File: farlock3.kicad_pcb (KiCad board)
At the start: 2 copper layers, 53 x 17.8 mm, 38 parts, among them J1 USB_B_Micro, J2 Conn_01x17, SW1 SW_SPDT, U1 MDBT50Q, U2 MX25R6435FZNIL0, U3 TB6612FNG, U4 AP2112K-3.3, Y1 32.768kHz

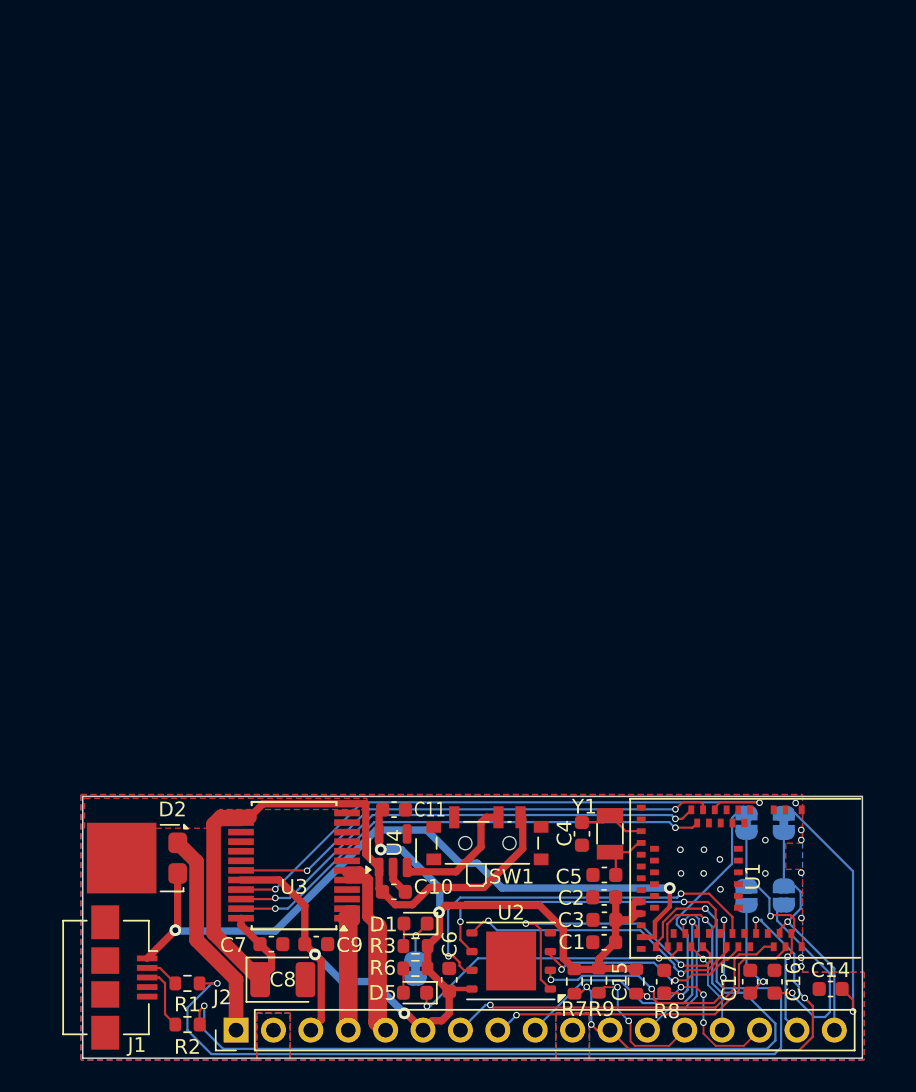
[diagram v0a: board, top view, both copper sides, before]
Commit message: v02 redesign
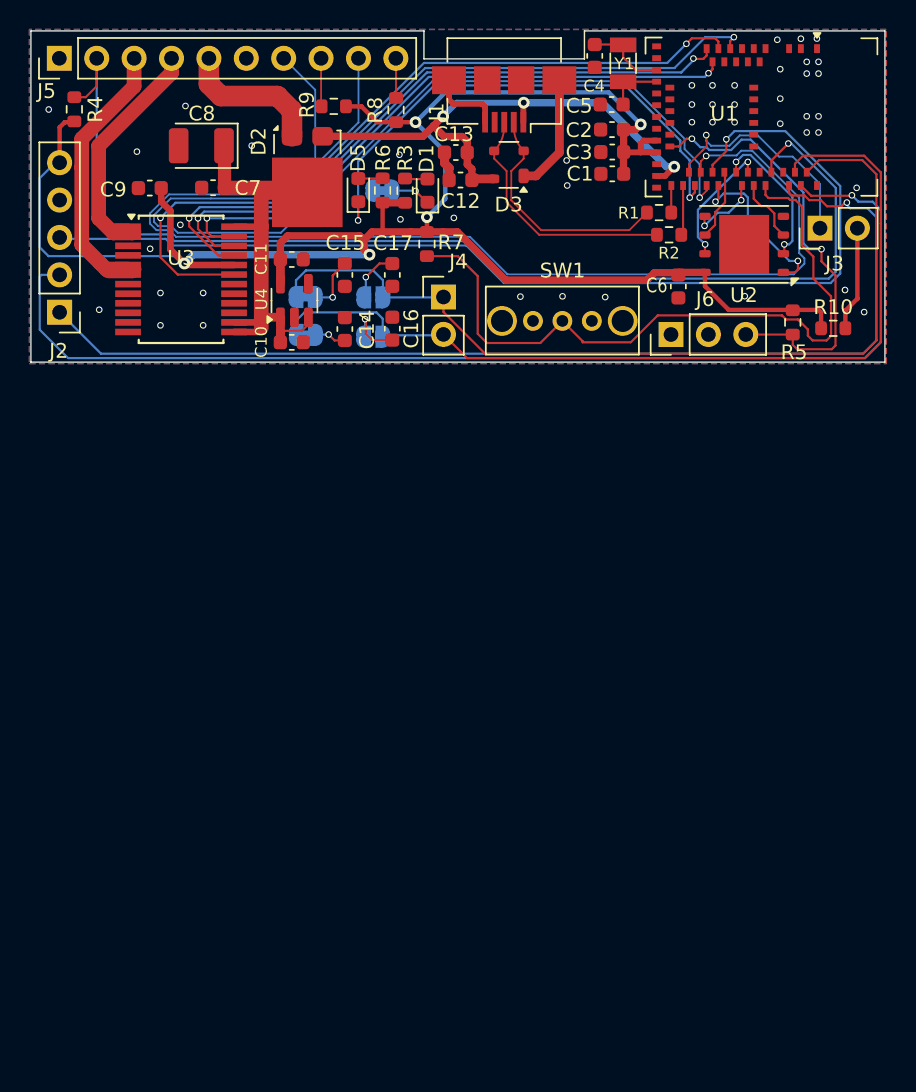
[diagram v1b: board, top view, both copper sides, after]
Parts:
- added C12: 10µF, Capacitor_SMD:C_0603_1608Metric, F.Cu at (155.6, 85.1)
- added C13: 0.1µF, Capacitor_SMD:C_0603_1608Metric, F.Cu at (155.3, 83.3)
- added D3: PRTR5V0U2X, Package_TO_SOT_SMD:SOT-143, F.Cu at (158.9, 84.1)
- added J3: Conn_01x02, Connector_PinHeader_2.54mm:PinHeader_1x02_P2.54mm_Vertical, F.Cu at (180.0, 88.4)
- added J4: Conn_01x02, Connector_PinHeader_2.54mm:PinHeader_1x02_P2.54mm_Vertical, F.Cu at (154.4, 93.1)
- added J5: Conn_01x10, Connector_PinHeader_2.54mm:PinHeader_1x10_P2.54mm_Vertical, F.Cu at (128.3, 76.9)
- added J6: Conn_01x03, Connector_PinHeader_2.54mm:PinHeader_1x03_P2.54mm_Vertical, F.Cu at (169.9, 95.6)
- added R10: 330, Resistor_SMD:R_0603_1608Metric, F.Cu at (180.9, 95.2)
- added R4: 10k, Resistor_SMD:R_0603_1608Metric, F.Cu at (129.3, 80.3)
- added R5: 10k, Resistor_SMD:R_0603_1608Metric, F.Cu at (178.2, 94.8)
- J2: value Conn_01x17 -> Conn_01x05; footprint Connector_PinHeader_2.54mm:PinHeader_1x17_P2.54mm_Vertical -> Connector_PinHeader_2.54mm:PinHeader_1x05_P2.54mm_Vertical
- SW1: footprint Button_Switch_SMD:SW_SPDT_PCM12 -> OS102011MA1QN1:OS102011MA1QN1
- U1: footprint MDBT50Q:MDBT50Q -> MDBT50Q:MDBT50Q-U1M
- moved J1 65.0 mm to (158.6, 79.7), turned to 180 degrees
- moved R2 62.8 mm to (169.8, 88.8)
- moved R9 62.1 mm to (147.0, 80.1), turned to 180 degrees
- moved R8 61.4 mm to (151.2, 80.4), turned to 90 degrees
- moved R1 61.4 mm to (169.1, 87.3)
- moved C8 56.9 mm to (138.0, 82.8), turned to 180 degrees
- moved C14 55.7 mm to (147.7, 95.2), turned to 90 degrees
- moved D5 54.7 mm to (148.6, 85.8), turned to 90 degrees
- moved C17 53.8 mm to (150.9, 91.6), turned to -90 degrees
- moved JP1 52.9 mm to (150.3, 85.8), turned to 0 degrees
- moved R6 52.9 mm to (150.3, 85.8), turned to 90 degrees
- moved C4 52.8 mm to (164.7, 76.7)
- moved C15 52.7 mm to (147.7, 91.6), turned to -90 degrees
- moved C9 52.6 mm to (134.5, 85.7), turned to 180 degrees
- moved Y1 52.3 mm to (166.6, 77.2)
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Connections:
- net D+_CON renamed D+
- net D-_CON renamed D-
- C1 pad 2: SW_POS2 -> GND
- C10 pad 2: SW_POS2 -> GND
- C11 pad 2: SW_POS2 -> GND
- C14 pad 2: SW_POS2 -> GND
- C15 pad 2: SW_POS2 -> GND
- C16 pad 2: SW_POS2 -> GND
- C17 pad 2: SW_POS2 -> GND
- C2 pad 2: SW_POS2 -> GND
- C3 pad 2: SW_POS2 -> GND
- C4 pad 2: SW_POS2 -> GND
- C5 pad 2: SW_POS2 -> GND
- C6 pad 2: SW_POS2 -> GND
- C7 pad 2: SW_POS2 -> GND
- C8 pad 2: SW_POS2 -> GND
- C9 pad 2: SW_POS2 -> GND
- J1 pad 5: SW_POS2 -> GND
- J1 pad 6: SW_POS2 -> GND
- J2 pad 1: VIN -> SWDIO
- J2 pad 2: SW_POS2 -> SWDCLK
- J2 pad 3: +3V3 -> RESET
- J2 pad 4: MOTOR_1 -> GND
- J2 pad 5: MOTOR_2 -> +3V3
- JP1 pad 1: SW_POS2 -> GND
- R7 pad 1: P0.25 -> P0.24
- SW1 pad 1: SW_POS2 -> unconnected-(SW1-A-Pad1)
- SW1 pad 2: Net-(SW1-B) -> P0.24
- SW1 pad 3: +VDC -> GND
- U1 pad 1: SW_POS2 -> GND
- U1 pad 15: SW_POS2 -> GND
- U1 pad 2: SW_POS2 -> GND
- U1 pad 29: unconnected-(U1-P0.12-Pad29) -> P0.12
- U1 pad 33: SW_POS2 -> GND
- U1 pad 36: unconnected-(U1-P0.14-Pad36) -> LED_CXN-
- U1 pad 48: unconnected-(U1-P0.24-Pad48) -> P0.24
- U1 pad 55: SW_POS2 -> GND
- U2 pad 4: SW_POS2 -> GND
- U3 pad 10: SW_POS2 -> GND
- U3 pad 18: SW_POS2 -> GND
- U3 pad 3: SW_POS2 -> GND
- U3 pad 4: SW_POS2 -> GND
- U3 pad 9: SW_POS2 -> GND
- U4 pad 2: SW_POS2 -> GND
- U4 pad 3: Net-(SW1-B) -> +VDC
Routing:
- net LED_ACCD-: track 13.1 -> 81.1 mm
- net Net-(U1-D-): track 65.5 -> 1.84 mm, vias 2 -> 0
- net LED_ACCG-: track 6.80 -> 69.0 mm
- net +3V3: track 70.6 -> 130.6 mm, vias 4 -> 5
- net SWDCLK: track 23.0 -> 78.5 mm
- net Net-(U1-D+): track 58.2 -> 3.44 mm, vias 2 -> 0
- net RESET: track 18.9 -> 72.7 mm
- net P0.25: track 30.5 -> 79.2 mm, vias 4 -> 1
- net P0.24: track 0.00 -> 48.4 mm
- net SWDIO: track 24.9 -> 72.8 mm
- net P0.09/NFC1: track 17.1 -> 62.0 mm, vias 1 -> 0
- net P0.10/NFC2: track 17.2 -> 61.6 mm, vias 2 -> 0
- net P0.12: track 0.00 -> 30.2 mm, vias 0 -> 2
- net P0.23: track 26.8 -> 8.63 mm
- net P0.19: track 22.9 -> 4.85 mm, vias 2 -> 0
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- added copper zone on B.Cu, net GND
- added copper zone on F.Cu, net GND
- removed copper zone on F.Cu, net +VDC
- removed copper zone on B.Cu, net SW_POS2
- removed copper zone on F.Cu, net SW_POS2
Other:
- board size 53 x 17.8 mm -> 58 x 22.5 mm
- board text added: "farlock3 v02"
- board text removed: "farlock3 v01"
